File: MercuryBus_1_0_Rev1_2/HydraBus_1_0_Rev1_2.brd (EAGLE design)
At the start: 60 x 37 mm, 60 parts, among them IC1 STM32F405RGT, J1 CON_HEADER_2X06, J2 CON_HEADER_2X08, J3 CON_HEADER_2X08, J4 MICRO-SDCARD-CONNECTOR-330006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, J5 CON_HEADER_1X06-PTH, U1 IP4220CZ6, Y1_8MHZ 631-1100-ND, Y2_32.768KHZ 32.768KHz

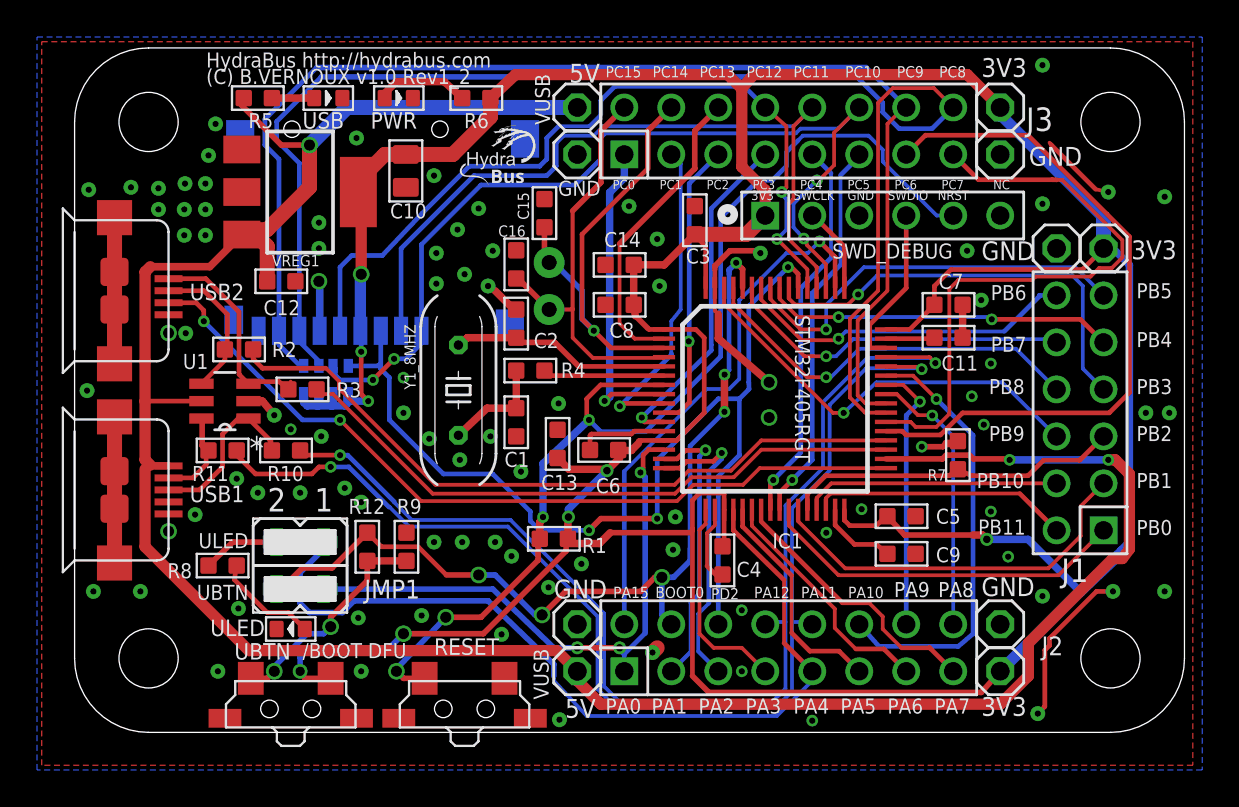
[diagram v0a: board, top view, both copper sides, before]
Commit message: Fourth commit
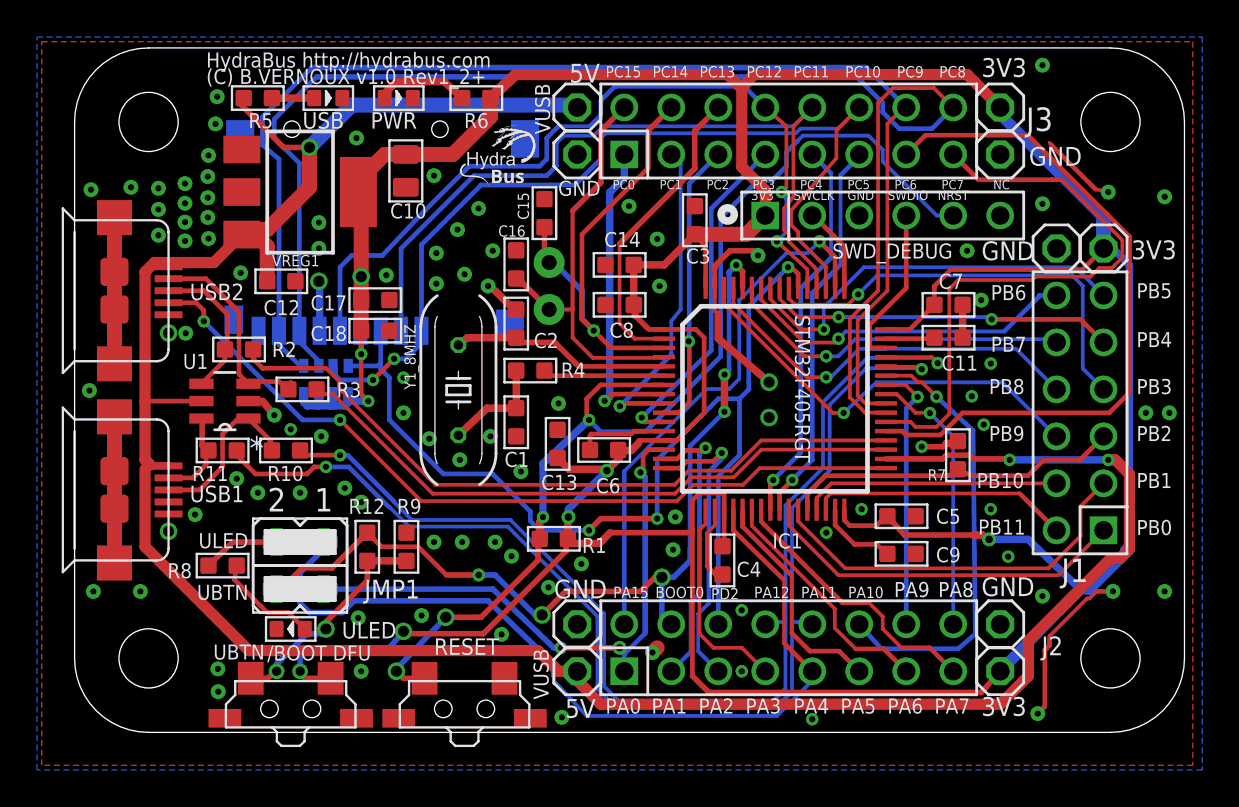
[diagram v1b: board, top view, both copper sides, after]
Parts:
- added C17: 1uF, OPL:C0603
- added C18: 100nF, OPL:C0603
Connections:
- net +3V3: now also C17.2, C18.1
- net GND: now also C17.1, C18.2
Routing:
- net +3V3: track 229.8 -> 234.9 mm
- net VUSB: track 137.5 -> 138.2 mm
- net GND: track 43.2 -> 42.6 mm, vias 91 -> 97
- net PC10: vias 4 -> 2
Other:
- board text added: "(C) B.VERNOUX v1.0 Rev1_2+"
- board text removed: "(C) B.VERNOUX v1.0 Rev1_2"
- board text removed: "SPI2_MOSI"
